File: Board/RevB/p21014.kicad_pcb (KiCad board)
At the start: 2 copper layers, 59.6 x 25.4 mm, 29 parts, among them J1 Conn_01x06_Male, J3 Conn_02x03_Counter_Clockwise, J4 Conn_01x08_Female, J5 Conn_01x12_Female, J6 Conn_01x06_Female, SW1 SW_Push

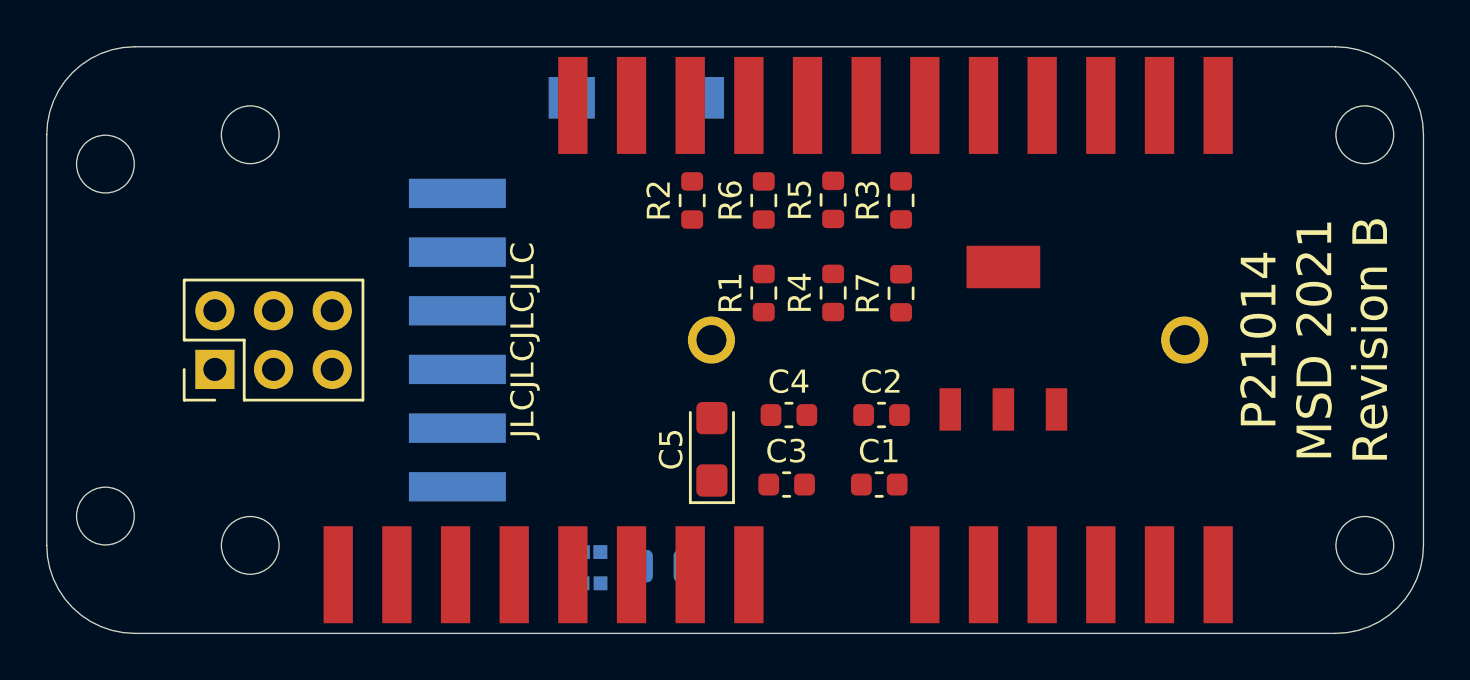
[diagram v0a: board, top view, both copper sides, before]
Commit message: Auto-routed RevB
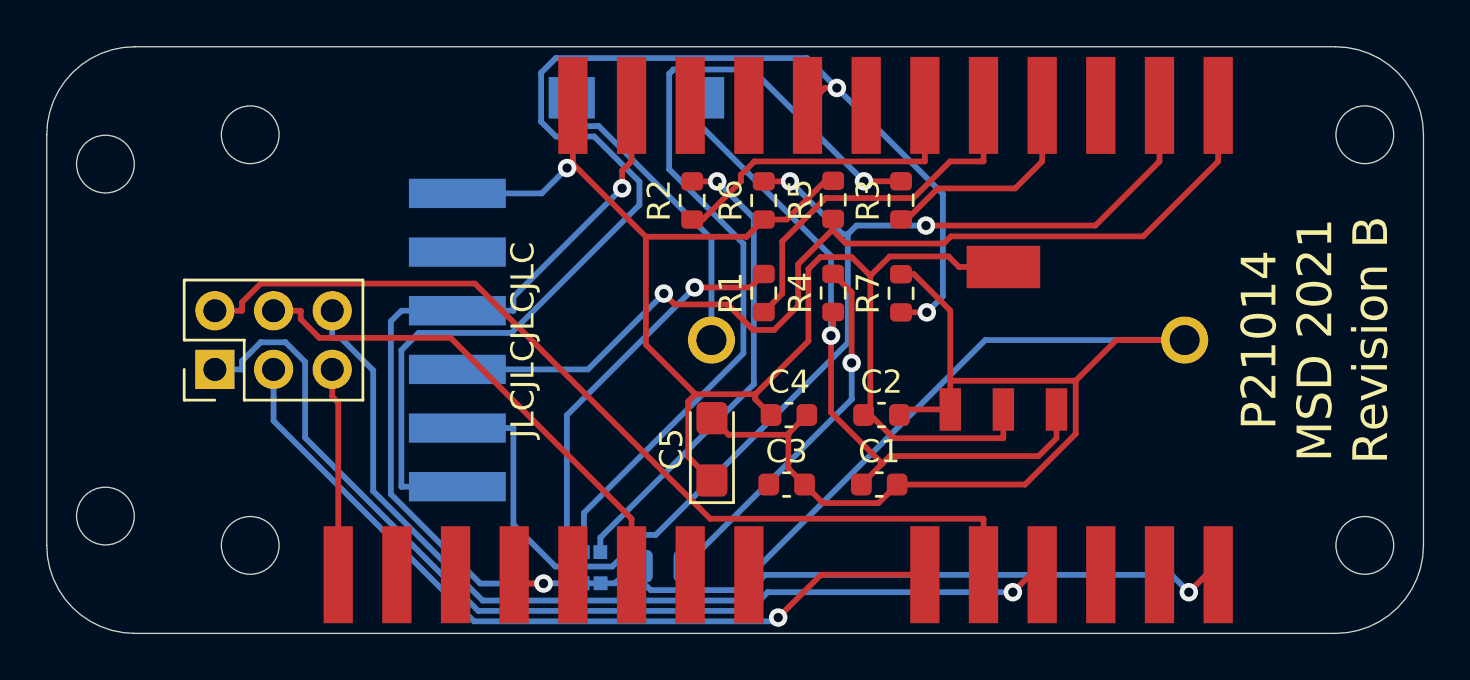
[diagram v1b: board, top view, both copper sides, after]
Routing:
- net GNDREF: track 0.00 -> 109.8 mm, vias 0 -> 2
- net +5V: track 0.00 -> 67.1 mm, vias 0 -> 1
- net /RST: track 0.00 -> 57.9 mm, vias 0 -> 2
- net /SCL: track 0.00 -> 52.5 mm, vias 0 -> 2
- net Net-(J3-Pad6): track 0.00 -> 48.4 mm, vias 0 -> 1
- net Net-(J3-Pad1): track 0.00 -> 43.9 mm, vias 0 -> 1
- net /SDA: track 0.00 -> 42.4 mm, vias 0 -> 1
- net Net-(J3-Pad2): track 0.00 -> 40.6 mm
- net Net-(D1-Pad2): track 0.00 -> 37.0 mm, vias 0 -> 1
- net Net-(J3-Pad3): track 0.00 -> 34.9 mm, vias 0 -> 1
- net +BATT: track 0.00 -> 30.7 mm, vias 0 -> 1
- net Net-(J3-Pad4): track 0.00 -> 21.9 mm
- net Net-(D1-Pad3): track 0.00 -> 20.5 mm, vias 0 -> 1
- net Net-(D1-Pad1): track 0.00 -> 17.0 mm, vias 0 -> 1
- net Net-(D2-Pad2): track 0.00 -> 16.0 mm, vias 0 -> 1
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
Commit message: Created RevB Gerber Files
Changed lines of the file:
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@@
       (drillshape 0)
       (scaleselection 1)
-      (outputdirectory "../##Gerber/RevA/"))
+      (outputdirectory "../##Gerber/RevB/"))
   )
   (net 0 "")
@@
       (effects (font (size 0.8 0.8) (thickness 0.12)))
     )
-    (pad 1 smd roundrect (at -1.35 0 90) (size 1.4 1.35) (layers F.Cu F.Paste F.Mask) (roundrect_rratio 0.185185)
+    (pad 1 smd roundrect (at -1.35 0 90) (size 1.4 1.35) (layers F.Cu F.Paste F.Mask) (roundrect_rratio 0.1851844444444445)
       (net 4 +5V))
-    (pad 2 smd roundrect (at 1.35 0 90) (size 1.4 1.35) (layers F.Cu F.Paste F.Mask) (roundrect_rratio 0.185185)
+    (pad 2 smd roundrect (at 1.35 0 90) (size 1.4 1.35) (layers F.Cu F.Paste F.Mask) (roundrect_rratio 0.1851844444444445)
       (net 1 GNDREF))
     (model ${KISYS3DMOD}/Capacitor_Tantalum_SMD.3dshapes/CP_EIA-3216-18_Kemet-A.wrl
